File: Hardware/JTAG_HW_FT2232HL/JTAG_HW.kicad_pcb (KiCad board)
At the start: 2 copper layers, 38 x 20.7 mm, 38 parts, among them J2 Conn_01x06_Male, J3 Conn_01x06_Male, J6 USB_C16PIN, U1 93CxxC, U2 AMS1117-3.3, U3 NUP2202, U4 FT2232HL, Y1 12MHZ

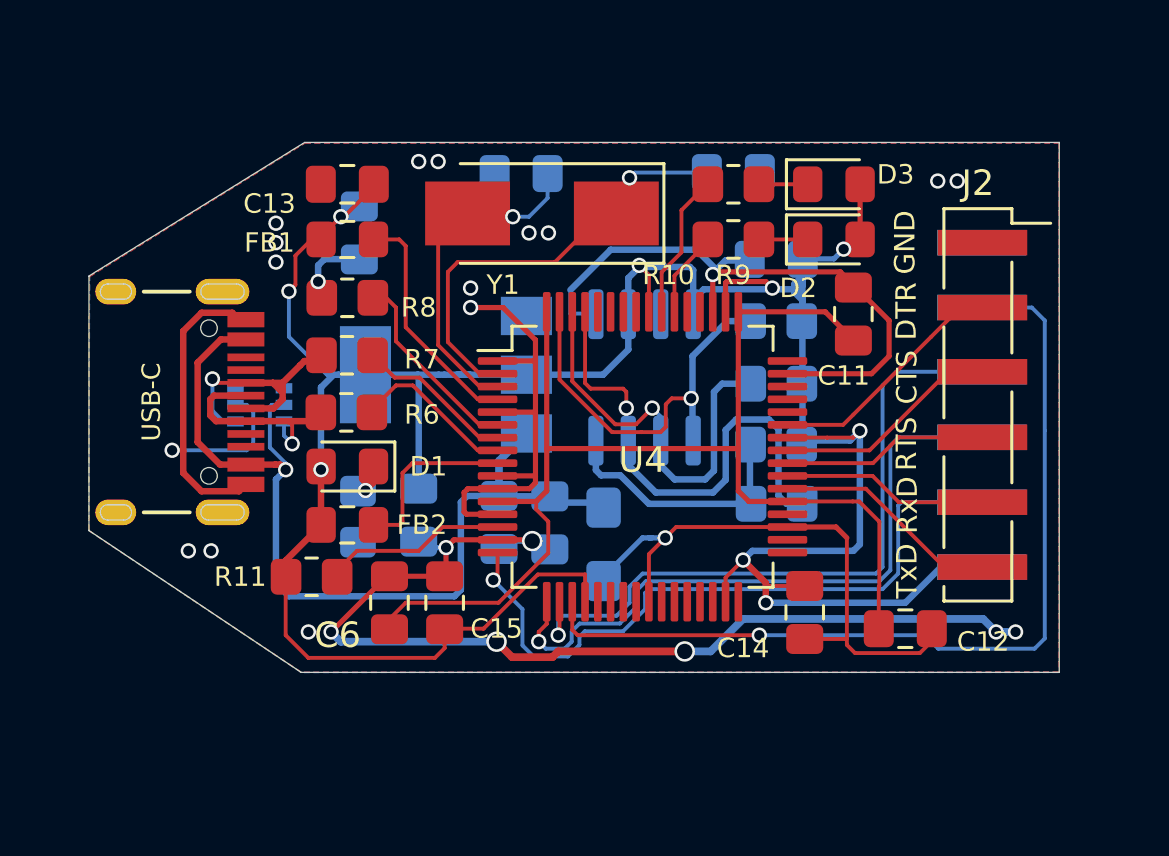
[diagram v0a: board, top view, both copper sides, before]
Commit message: Retrace pcb. Add some tips
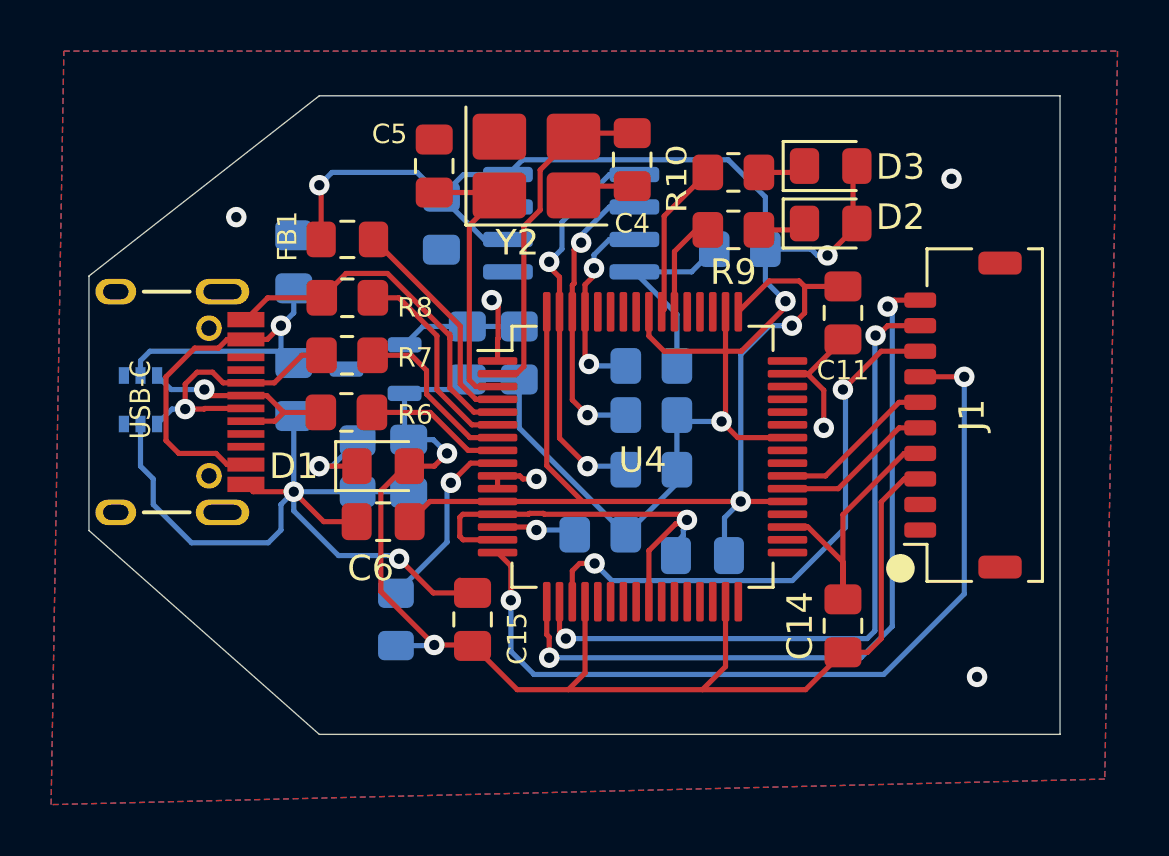
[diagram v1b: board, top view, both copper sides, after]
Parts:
- removed C10: 10uF, Capacitor_Tantalum_SMD:CP_EIA-3216-18_Kemet-A_Pad1.58x1.35mm_HandSolder
- removed J2, J3: Conn_01x06_Male, JTAG_HW:PinHeader_1x06_P2.54mm_Vertical_SMD_Pin1long
- removed U2: AMS1117-3.3, Package_TO_SOT_SMD:SOT-223-3_TabPin2
- removed Y1: 12MHZ, Crystal:Crystal_SMD_0603-2Pin_6.0x3.5mm_HandSoldering
- added J1: Conn_01x10_Pin, Connector_JST:JST_SHL_SM10B-SHLS-TF_1x10-1MP_P1.00mm_Horizontal, F.Cu at (165.2, 102.0)
- added U5: XC6206PxxxMR, Package_TO_SOT_SMD:SOT-23-3, B.Cu at (142.2, 100.2)
- added Y2: Crystal_GND24, Crystal:Crystal_SMD_3225-4Pin_3.2x2.5mm_HandSoldering, F.Cu at (148.5, 92.2)
- C12, C13, FB2, R11: moved to B.Cu
- C4, C5: moved to F.Cu
- moved C9 14.3 mm to (139.0, 96.0), turned to 90 degrees
- moved C1 13.2 mm to (144.8, 94.5), turned to -90 degrees
- moved R11 11.4 mm to (151.0, 106.7), turned to 180 degrees
- moved C2 9.57 mm to (139.0, 101.0)
- moved C13 9.43 mm to (147.8, 99.6), turned to 90 degrees
- moved C12 8.44 mm to (155.0, 107.5), turned to 180 degrees
- moved R3 7.78 mm to (156.5, 95.5)
- moved R1 7.60 mm to (153.0, 104.1)
- moved R4 7.29 mm to (153.0, 100.1)
- moved U1 6.69 mm to (149.9, 94.5), turned to 180 degrees
- moved C7 6.32 mm to (145.8, 99.6), turned to 90 degrees
- moved R2 5.04 mm to (153.0, 102.0)
- moved U3 4.67 mm to (133.0, 101.4), turned to 90 degrees
- moved FB2 4.16 mm to (143.0, 110.0), turned to -90 degrees
- moved C4 3.99 mm to (152.2, 92.0), turned to -90 degrees
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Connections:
- net +3V3 renamed 3.3V
- J6 pad A5: (no net) -> unconnected-(J6-CC1-PadA5)
- J6 pad B5: (no net) -> unconnected-(J6-CC2-PadB5)
- R3 pad 1: Net-(R3-Pad1) -> Net-(U1-DO)
- R4 pad 1: Net-(R3-Pad1) -> Net-(U1-DI)
- R4 pad 2: Net-(R4-Pad2) -> Net-(U1-DO)
- U1 pad 3: Net-(R4-Pad2) -> Net-(U1-DI)
- U1 pad 4: Net-(R3-Pad1) -> Net-(U1-DO)
- U1 pad 7: (no net) -> unconnected-(U1-NC-Pad7)
- U3 pad 3: (no net) -> unconnected-(U3-Pad3)
- U3 pad 4: (no net) -> unconnected-(U3-Pad4)
- U4 pad 21: (no net) -> unconnected-(U4-ADBUS4-Pad21)
- U4 pad 22: (no net) -> unconnected-(U4-ADBUS5-Pad22)
- U4 pad 23: (no net) -> unconnected-(U4-ADBUS6-Pad23)
- U4 pad 24: (no net) -> unconnected-(U4-ADBUS7-Pad24)
- U4 pad 26: (no net) -> unconnected-(U4-ACBUS0-Pad26)
- U4 pad 27: (no net) -> unconnected-(U4-ACBUS1-Pad27)
- U4 pad 28: (no net) -> unconnected-(U4-ACBUS2-Pad28)
- U4 pad 29: (no net) -> unconnected-(U4-ACBUS3-Pad29)
- U4 pad 30: (no net) -> unconnected-(U4-ACBUS4-Pad30)
- U4 pad 32: (no net) -> unconnected-(U4-ACBUS5-Pad32)
- U4 pad 33: (no net) -> unconnected-(U4-ACBUS6-Pad33)
- U4 pad 34: (no net) -> unconnected-(U4-ACBUS7-Pad34)
- U4 pad 36: (no net) -> unconnected-(U4-~{SUSPEND}-Pad36)
- U4 pad 44: (no net) -> unconnected-(U4-BDBUS5-Pad44)
- U4 pad 45: (no net) -> unconnected-(U4-BDBUS6-Pad45)
- U4 pad 46: (no net) -> unconnected-(U4-BDBUS7-Pad46)
- U4 pad 48: (no net) -> unconnected-(U4-BCBUS0-Pad48)
- U4 pad 52: (no net) -> unconnected-(U4-BCBUS1-Pad52)
- U4 pad 53: (no net) -> unconnected-(U4-BCBUS2-Pad53)
- U4 pad 57: (no net) -> unconnected-(U4-BCBUS5-Pad57)
- U4 pad 58: (no net) -> unconnected-(U4-BCBUS6-Pad58)
- U4 pad 59: (no net) -> unconnected-(U4-BCBUS7-Pad59)
- U4 pad 60: (no net) -> unconnected-(U4-~{PWREN}-Pad60)
- U4 pad 61: Net-(R4-Pad2) -> Net-(U1-DI)
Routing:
- net GND: track 128.9 -> 93.7 mm, vias 25 -> 9
- net Net-(R4-Pad2): track 19.9 -> 0.00 mm, vias 1 -> 0
- net +5V: track 37.6 -> 24.0 mm
- net /TMS: track 35.4 -> 22.3 mm, vias 1 -> 2
- net Net-(R3-Pad1): track 10.1 -> 0.00 mm
- net /DTR: track 9.69 -> 0.00 mm
- net +1V8: track 48.7 -> 39.7 mm, vias 0 -> 2
- net /CTS: track 8.80 -> 0.00 mm
- net /RTS: track 8.08 -> 0.00 mm
- net Net-(U1-DO): track 0.00 -> 7.87 mm
- net Net-(U1-DI): track 0.00 -> 7.85 mm, vias 0 -> 2
- net /TCK: track 27.0 -> 33.7 mm, vias 1 -> 2
- net Net-(U1-SCLK): track 16.3 -> 11.5 mm, vias 1 -> 2
- net Net-(U4-OSCI): track 17.9 -> 13.3 mm, vias 1 -> 0
- net Net-(U4-~{RESET}): track 7.48 -> 3.14 mm, vias 0 -> 1
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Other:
- board size 38 x 20.7 mm -> 38 x 25 mm
- net class Default removed
- net class Pow-1.0A removed
- net class Pow-1.5A removed
- net class Pow-2.0A removed
- net class Pow-3.0A removed
- net class Pow-5.0A removed
- rule pad_to_mask_clearance: 0.051 -> 0
- board text removed: "3v3"
- board text removed: "CTS"
- board text removed: "DTR"
- board text removed: "GND"
- board text removed: "RTS"
- board text removed: "RxD"
- board text removed: "TCK"
- board text removed: "TDI"
- board text removed: "TDO"
- board text removed: "TMS"
- board text removed: "TxD"
